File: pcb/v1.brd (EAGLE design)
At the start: 92 x 80 mm, 61 parts, among them T1 MMBT3904, T2 MMBT3904, T3 MMBT3904, T4 MMBT3904

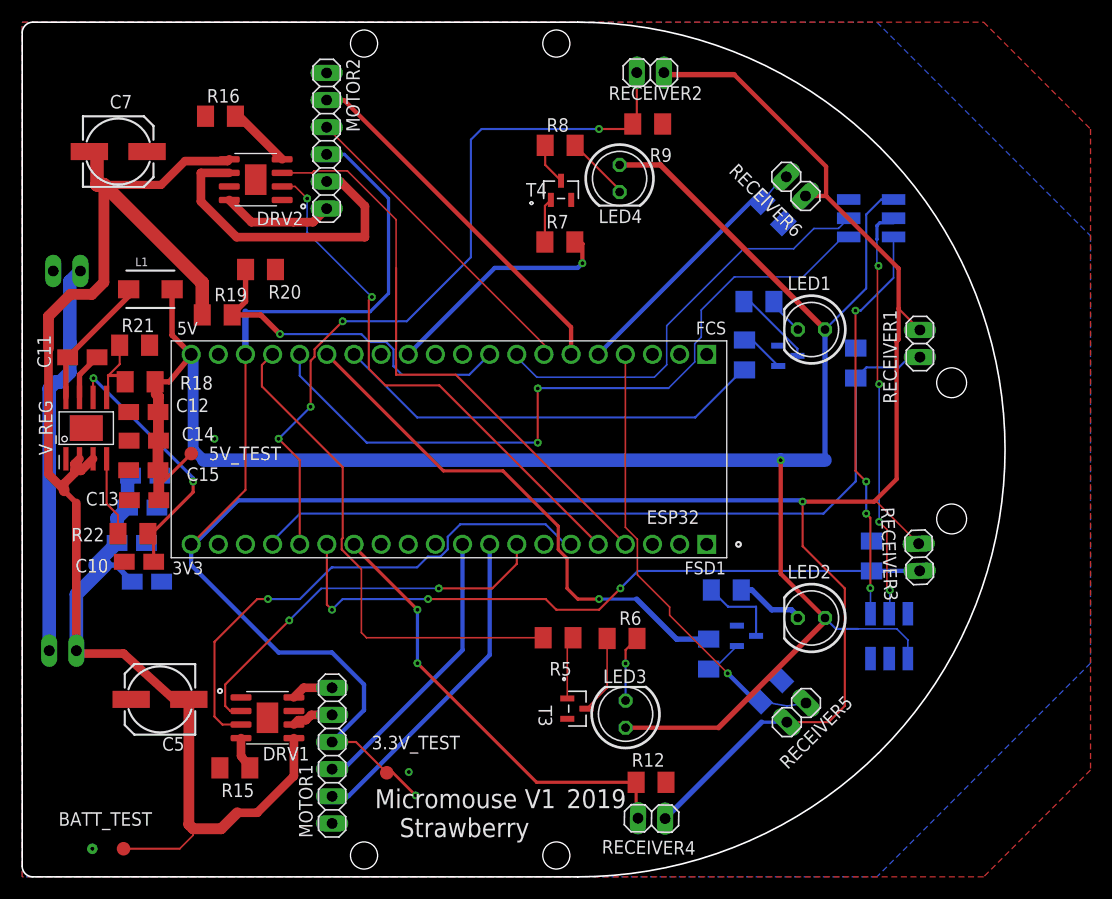
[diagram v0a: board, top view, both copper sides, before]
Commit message: Added Strawberry
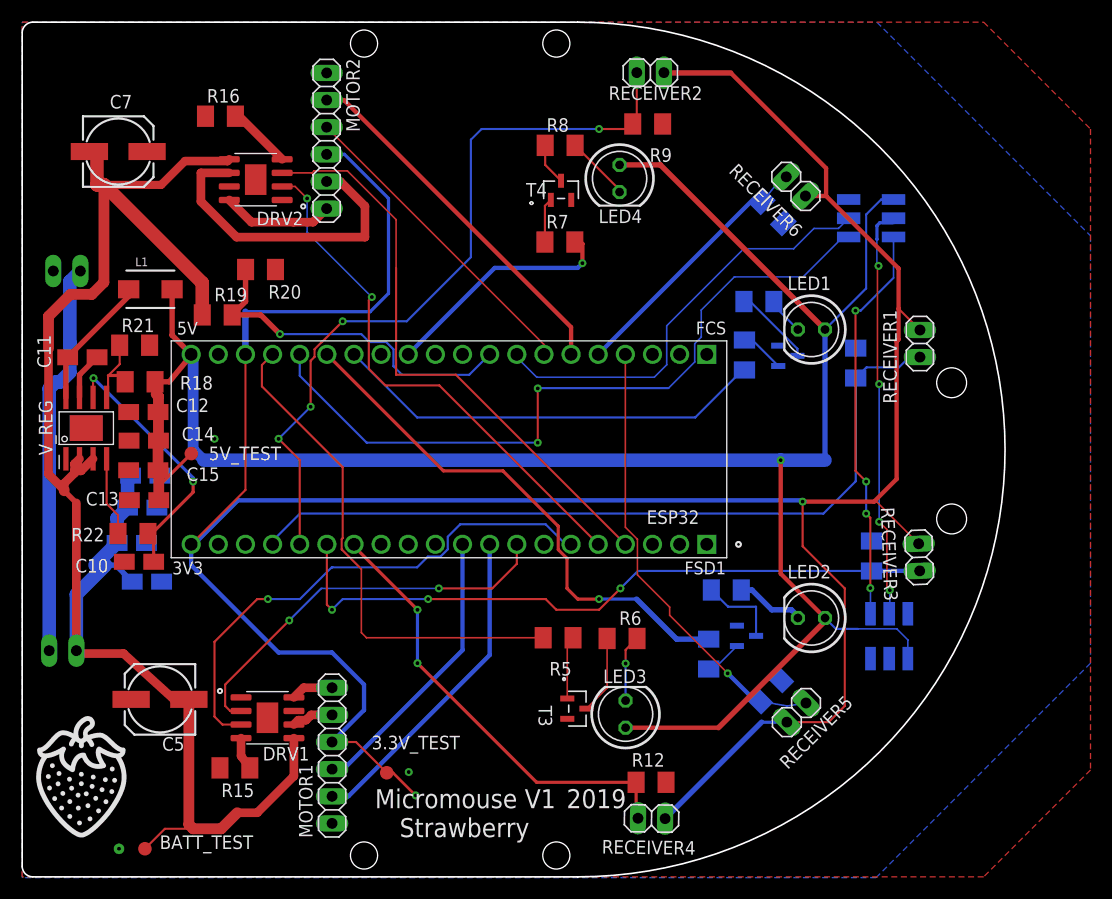
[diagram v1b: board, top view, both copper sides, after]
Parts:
- moved BATT_TEST 2.00 mm to (11.5, 2.63)
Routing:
- net BATT_POWER: track 157.7 -> 155.3 mm
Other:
- board text added: "/Users/vamsighorakavi/Downloads/strawberry(2).bmp"
